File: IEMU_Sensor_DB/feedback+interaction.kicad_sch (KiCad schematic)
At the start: 28 parts, among them J301 Conn_01x02_Pin, M401 VZ43FM1B8230001L, Q301 CSD13381F4, Q302 CSD13381F4, Q303 CSD13381F4, Q304 CSD13381F4, SW301 NANOT_160_BP, SW302 TS-1088-AR02016

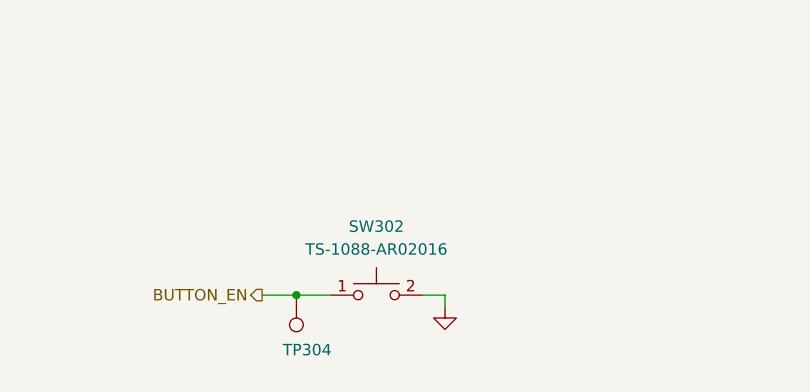
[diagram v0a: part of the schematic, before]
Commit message: commit after component purchase
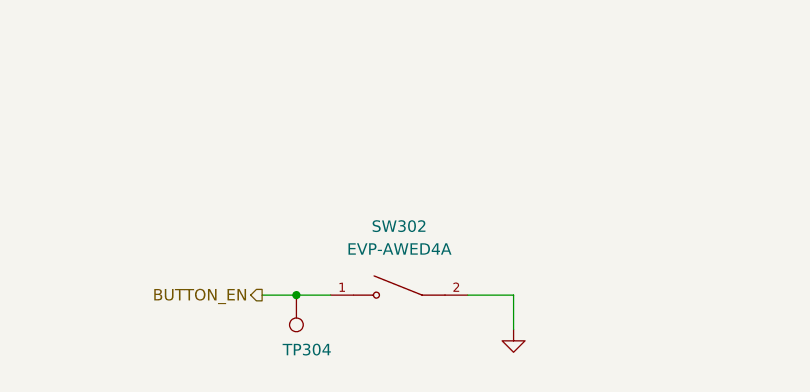
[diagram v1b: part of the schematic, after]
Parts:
- removed SW302: TS-1088-AR02016, 0_Feedback:SW_TS-1088-AR02016, symbol 0_Feedback:TS-1088-AR02016
- added SW302: EVP-AWED4A, 0_Feedback:SW_EVP-AWED4A, symbol 0_Feedback:EVP-AWED4A
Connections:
- net BUTTON_EN: now also SW302.1
- net GND: now also SW302.2
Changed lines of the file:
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@@
 	(wire
 		(pts
-			(xy 120.65 160.02) (xy 120.65 161.29)
-		)
-		(stroke
-			(width 0)
-			(type default)
-		)
-	)
-	(wire
-		(pts
 			(xy 104.14 102.87) (xy 104.14 91.44)
 		)
@@
 	(wire
 		(pts
-			(xy 118.11 160.02) (xy 120.65 160.02)
+			(xy 128.27 160.02) (xy 128.27 163.83)
+		)
+		(stroke
+			(width 0)
+			(type default)
+		)
+	)
+	(wire
+		(pts
+			(xy 123.19 160.02) (xy 128.27 160.02)
 		)
 		(stroke
@@
 	)
 	(symbol
-		(lib_id "0_Feedback:TS-1088-AR02016")
-		(at 113.03 160.02 0)
+		(lib_id "0_Power:D_Schottky_2A_40V_0603")
+		(at 110.49 86.36 270)
 		(unit 1)
 		(exclude_from_sim no)
@@
 		(on_board yes)
 		(dnp no)
-		(fields_autoplaced yes)
-		(property "Reference" "SW302"
-			(at 113.03 152.4 0)
-			(effects
-				(font
-					(size 1.27 1.27)
-				)
-			)
-		)
-		(property "Value" "TS-1088-AR02016"
-			(at 113.03 154.94 0)
+		(property "Reference" "D302"
+			(at 114.808 83.058 90)
 			(effects
 				(font
@@
 			)
 		)
-		(property "Footprint" "0_Feedback:SW_TS-1088-AR02016"
-			(at 113.03 167.132 0)
+		(property "Value" "D_Schottky_2A_40V_0603"
+			(at 113.284 86.868 0)
 			(effects
 				(font
 					(size 1.27 1.27)
 				)
-				(justify bottom)
 				(hide yes)
 			)
 		)
-		(property "Datasheet" "https://jlcpcb.com/api/file/downloadByFileSystemAccessId/8588886944068096000"
-			(at 113.03 166.37 0)
+		(property "Footprint" "0_Power:0603_DSN"
+			(at 110.49 86.36 0)
 			(effects
 				(font
@@
 			)
 		)
-		(property "Description" "50mA 4mm 100MΩ 100,000 Times 12V 160gf 3mm 2mm Round Button Vertical welding SPST SMD Tactile Switches ROHS"
-			(at 113.03 169.418 0)
+		(property "Datasheet" "https://jlcpcb.com/api/file/downloadByFileSystemAccessId/8588900416898158592"
+			(at 110.49 86.36 0)
 			(effects
 				(font
@@
 			)
 		)
-		(property "Manufacturer_Name" "Xunpu"
-			(at 113.03 169.418 0)
+		(property "Description" "1 Independent 150uA@40V 2A 40V 550mV@2A 0603 Schottky Diodes ROHS"
+			(at 110.49 86.36 0)
 			(effects
 				(font
 					(size 1.27 1.27)
 				)
-				(justify bottom)
 				(hide yes)
 			)
 		)
-		(property "Manufacturer_Part_Number" "TS-1088-AR02016"
-			(at 113.03 171.45 0)
+		(property "Manufacturer_Part_Number" "NSR20F40NXT5G"
+			(at 110.49 86.36 0)
 			(effects
 				(font
 					(size 1.27 1.27)
 				)
-				(justify bottom)
 				(hide yes)
 			)
 		)
-		(property "Distributor Link 1" ""
-			(at 113.03 160.02 0)
+		(property "Manufacturer_Name" "onsemi"
+			(at 110.49 86.36 0)
 			(effects
 				(font
 					(size 1.27 1.27)
 				)
-				(justify bottom)
 				(hide yes)
 			)
 		)
-		(property "Distributor Link 2" ""
-			(at 113.03 160.02 0)
+		(property "Distributor Link 1" "https://www.mouser.de/ProductDetail/onsemi/NSR20F40NXT5G?qs=Tr3lMbyRyKlnDYqqgtCWgQ%3D%3D"
+			(at 110.49 86.36 0)
 			(effects
 				(font
 					(size 1.27 1.27)
 				)
-				(justify bottom)
 				(hide yes)
 			)
 		)
-		(property "LCSC" "C720477"
-			(at 114.554 172.212 0)
+		(property "Distributor Link 2" "https://www.digikey.de/de/products/detail/onsemi/NSR20F40NXT5G/4848728?s=N4IgTCBcDaIHIGUBKYAMAxALKuANAKgKwDiIAugL5A"
+			(at 110.49 86.36 0)
 			(effects
 				(font
 					(size 1.27 1.27)
 				)
-				(justify bottom)
 				(hide yes)
 			)
 		)
-		(property "Distributer Link 1" ""
-			(at 113.03 160.02 0)
+		(property "LCSC" "C153761"
+			(at 110.49 86.36 0)
 			(effects
 				(font
@@
 		)
 		(property "Manufactuer_Name" ""
-			(at 113.03 160.02 0)
+			(at 110.49 86.36 90)
 			(effects
 				(font
@@
 		)
 		(instances
-			(project ""
+			(project "IEMU_Sensor_DB"
 				(path "/114b31f2-6a4f-42ef-aa97-5a200e091126/bedc77cc-dda1-48b8-87d2-cdf0a97ca477"
-					(reference "SW302")
+					(reference "D302")
 					(unit 1)
 				)
@@
 	)
 	(symbol
-		(lib_id "0_Power:D_Schottky_2A_40V_0603")
-		(at 110.49 86.36 270)
+		(lib_id "0_Feedback:EVP-AWED4A")
+		(at 115.57 160.02 0)
 		(unit 1)
 		(exclude_from_sim no)
@@
 		(on_board yes)
 		(dnp no)
-		(property "Reference" "D302"
-			(at 114.808 83.058 90)
-			(effects
-				(font
-					(size 1.27 1.27)
-				)
-			)
-		)
-		(property "Value" "D_Schottky_2A_40V_0603"
-			(at 113.284 86.868 0)
-			(effects
-				(font
-					(size 1.27 1.27)
-				)
-				(hide yes)
-			)
-		)
-		(property "Footprint" "0_Power:0603_DSN"
-			(at 110.49 86.36 0)
-			(effects
-				(font
-					(size 1.27 1.27)
-				)
-				(hide yes)
-			)
-		)
-		(property "Datasheet" "https://jlcpcb.com/api/file/downloadByFileSystemAccessId/8588900416898158592"
-			(at 110.49 86.36 0)
-			(effects
-				(font
-					(size 1.27 1.27)
-				)
-				(hide yes)
-			)
-		)
-		(property "Description" "1 Independent 150uA@40V 2A 40V 550mV@2A 0603 Schottky Diodes ROHS"
-			(at 110.49 86.36 0)
+		(fields_autoplaced yes)
+		(property "Reference" "SW302"
+			(at 115.57 152.4 0)
 			(effects
 				(font
 					(size 1.27 1.27)
 				)
-				(hide yes)
 			)
 		)
-		(property "Manufacturer_Part_Number" "NSR20F40NXT5G"
-			(at 110.49 86.36 0)
+		(property "Value" "EVP-AWED4A"
+			(at 115.57 154.94 0)
 			(effects
 				(font
 					(size 1.27 1.27)
 				)
-				(hide yes)
 			)
 		)
-		(property "Manufacturer_Name" "onsemi"
-			(at 110.49 86.36 0)
+		(property "Footprint" "0_Feedback:SW_EVP-AWED4A"
+			(at 115.57 155.194 0)
 			(effects
 				(font
 					(size 1.27 1.27)
 				)
+				(justify bottom)
 				(hide yes)
 			)
 		)
-		(property "Distributor Link 1" "https://www.mouser.de/ProductDetail/onsemi/NSR20F40NXT5G?qs=Tr3lMbyRyKlnDYqqgtCWgQ%3D%3D"
-			(at 110.49 86.36 0)
+		(property "Datasheet" "https://mm.digikey.com/Volume0/opasdata/d220001/medias/docus/8810/sw_lt_eng_3020s.pdf"
+			(at 115.57 165.862 0)
 			(effects
 				(font
@@
 			)
 		)
-		(property "Distributor Link 2" "https://www.digikey.de/de/products/detail/onsemi/NSR20F40NXT5G/4848728?s=N4IgTCBcDaIHIGUBKYAMAxALKuANAKgKwDiIAugL5A"
-			(at 110.49 86.36 0)
+		(property "Description" "Tactile Switch SPST-NO Top Actuated Surface Mount"
+			(at 117.348 152.4 0)
 			(effects
 				(font
@@
 			)
 		)
-		(property "LCSC" "C153761"
-			(at 110.49 86.36 0)
+		(property "Manufacturer_Name" "Panasonic"
+			(at 115.57 169.164 0)
 			(effects
 				(font
 					(size 1.27 1.27)
 				)
+				(justify bottom)
 				(hide yes)
 			)
 		)
-		(property "Manufactuer_Name" ""
-			(at 110.49 86.36 90)
+		(property "Manufacturer_Part_Number" "EVP-AWBD2A"
+			(at 115.57 173.482 0)
 			(effects
 				(font
 					(size 1.27 1.27)
 				)
+				(justify bottom)
 				(hide yes)
 			)
@@
 		)
 		(instances
-			(project "IEMU_Sensor_DB"
+			(project ""
 				(path "/114b31f2-6a4f-42ef-aa97-5a200e091126/bedc77cc-dda1-48b8-87d2-cdf0a97ca477"
-					(reference "D302")
+					(reference "SW302")
 					(unit 1)
 				)
@@
 	(symbol
 		(lib_id "power:GND")
-		(at 120.65 161.29 0)
+		(at 128.27 163.83 0)
 		(mirror y)
 		(unit 1)
@@
 		(fields_autoplaced yes)
 		(property "Reference" "#PWR063"
-			(at 120.65 167.64 0)
+			(at 128.27 170.18 0)
 			(effects
 				(font
@@
 		)
 		(property "Value" "GND"
-			(at 120.65 165.1 0)
+			(at 128.27 167.64 0)
 			(effects
 				(font
@@
 		)
 		(property "Footprint" ""
-			(at 120.65 161.29 0)
+			(at 128.27 163.83 0)
 			(effects
 				(font
@@
 		)
 		(property "Datasheet" ""
-			(at 120.65 161.29 0)
+			(at 128.27 163.83 0)
 			(effects
 				(font
@@
 		)
 		(property "Description" "Power symbol creates a global label with name \"GND\" , ground"
-			(at 120.65 161.29 0)
+			(at 128.27 163.83 0)
 			(effects
 				(font
